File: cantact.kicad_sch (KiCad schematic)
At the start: 37 parts, among them P1 USB, P2 SWD, P3 DB9, U1 STM32F042C6T6, U2 AAT3221, U3 MCP2551-I/SN, X1 16 MHz

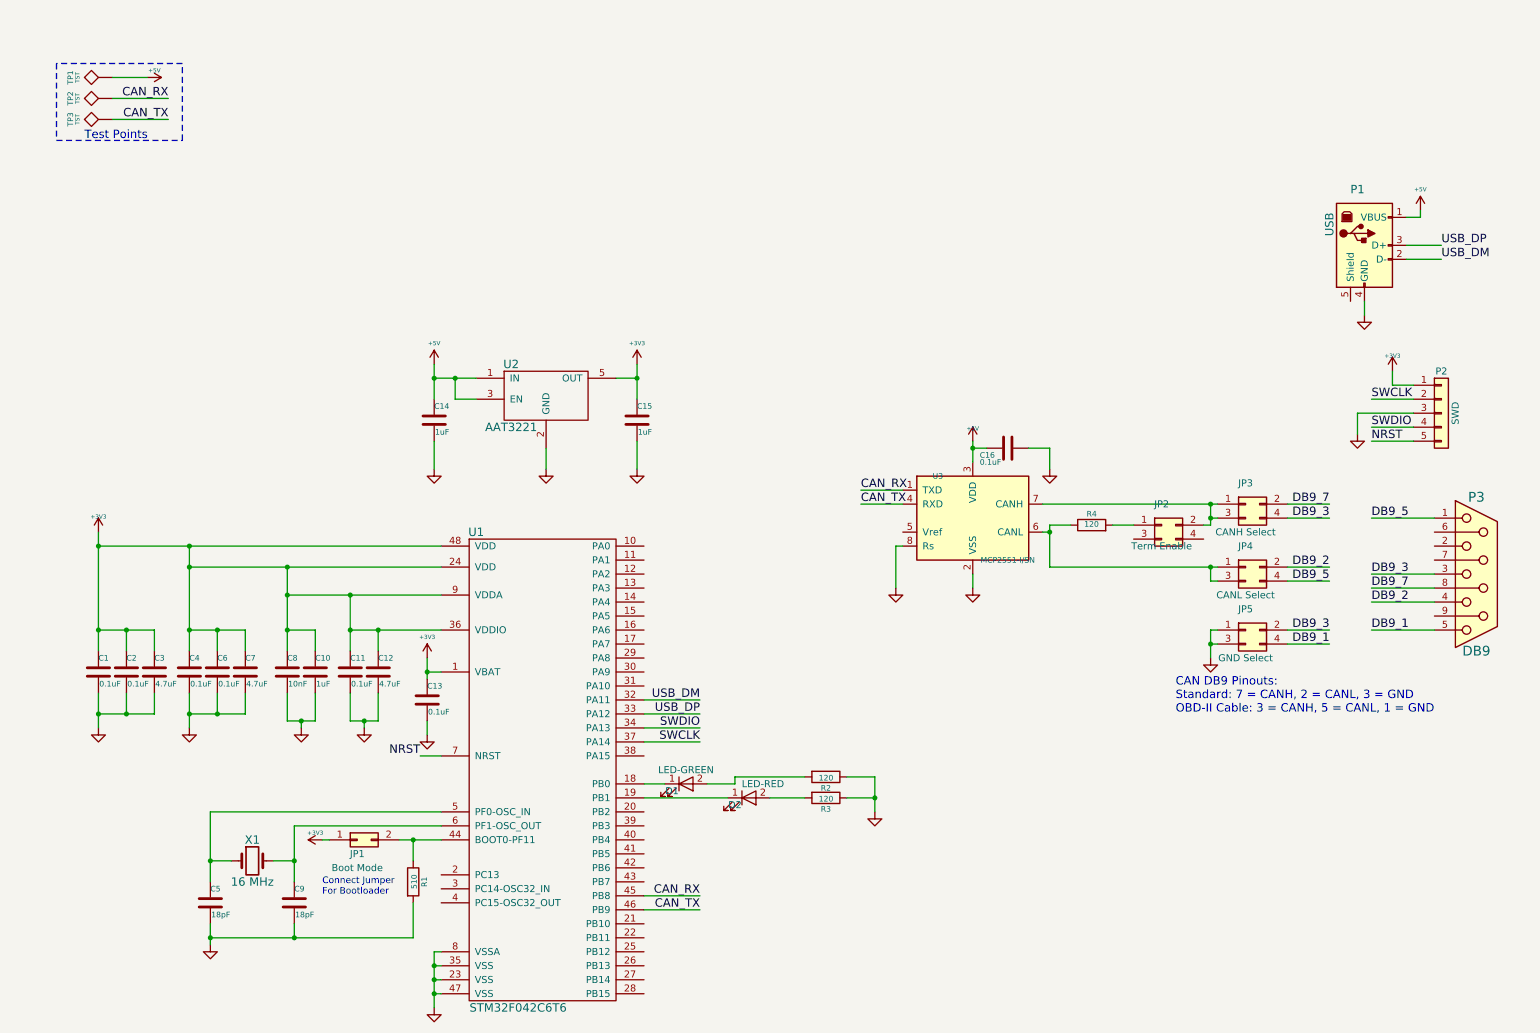
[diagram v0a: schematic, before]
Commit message: feat(hw):  schematic & pcb updated
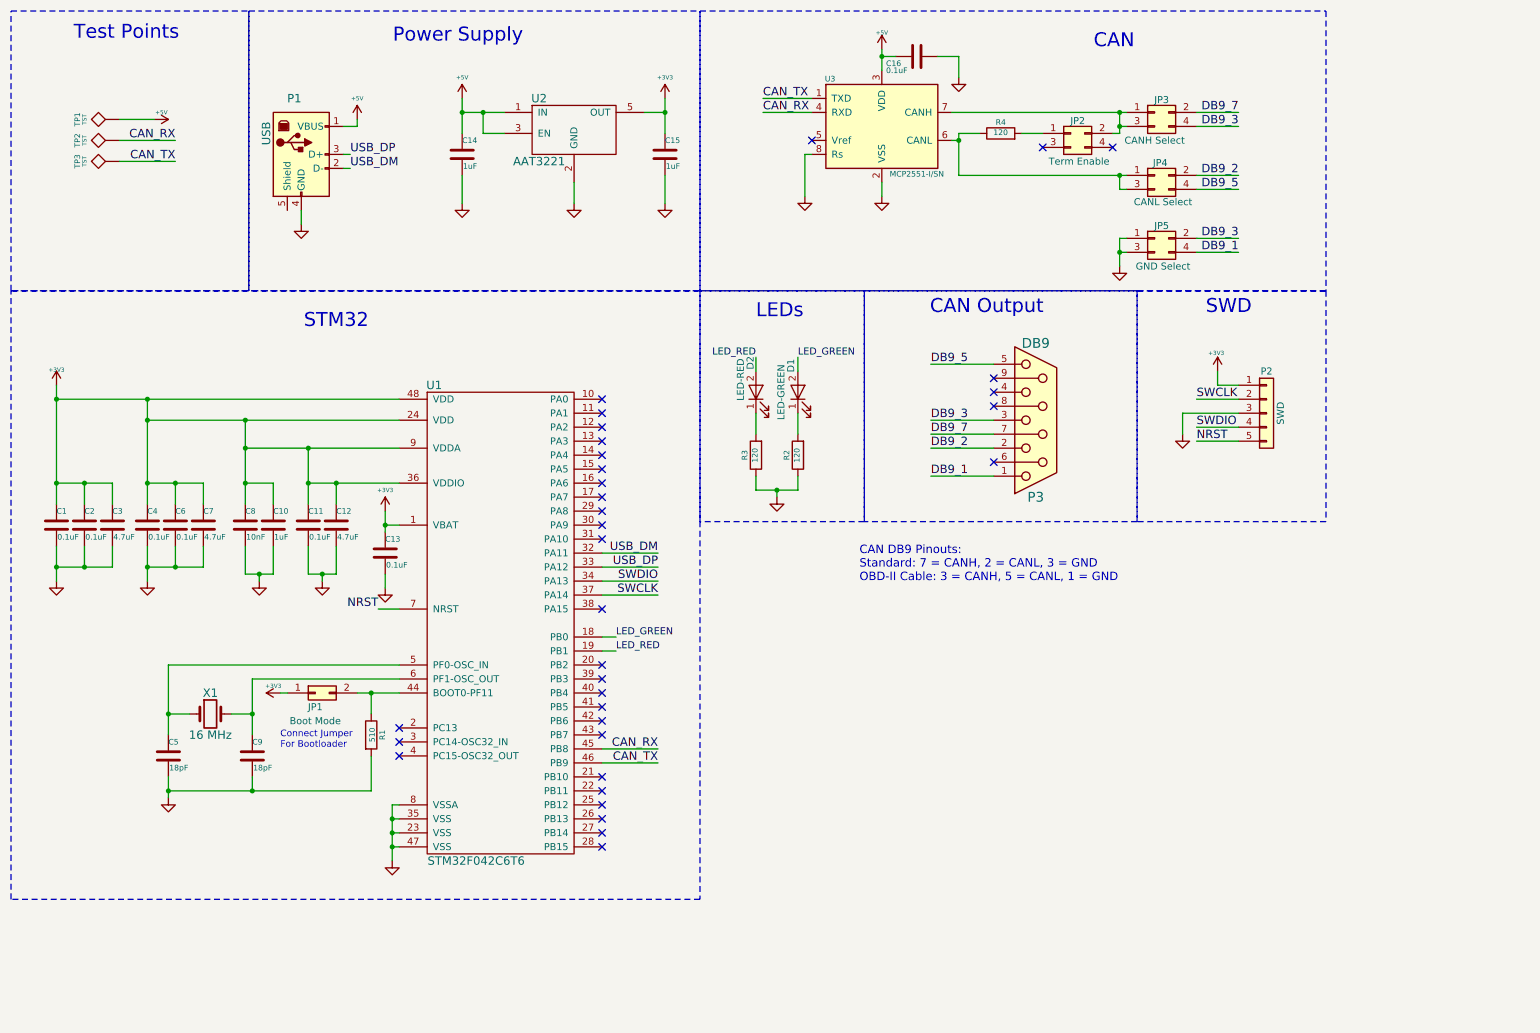
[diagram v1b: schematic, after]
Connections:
- net CAN_RX: now also U3.4 (RXD); no longer U3.1 (TXD)
- net CAN_TX: now also U3.1 (TXD); no longer U3.4 (RXD)
- net DB9_1: now also P3.1; no longer P3.5
- net DB9_2: now also P3.2; no longer P3.4
- net DB9_5: now also P3.5; no longer P3.1
- net DB9_7: now also P3.7; no longer P3.8
- net at D1.1 (K): now also R2.2; no longer U1.18 (PB0)
- net at D2.1 (K): now also R3.2; no longer U1.19 (PB1)
- net LED_GREEN: now reaches D1.2 (A)
- net LED_GREEN: now also U1.18 (PB0); no longer R2.2
- net LED_RED: now reaches D2.2 (A)
- net LED_RED: now also U1.19 (PB1); no longer R3.2
- no-connect marks 0 -> 34
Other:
- note added: "CAN"
- note added: "CAN Output"
- note added: "LEDs"
- note added: "Power Supply"
- note added: "STM32"
- note added: "SWD"
- moved on the sheet: C1, C10, C11, C12, C13, C14, C15, C16, C2, C3, C4, C5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
